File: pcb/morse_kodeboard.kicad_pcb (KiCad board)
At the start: 2 copper layers, 40 x 24 mm, 7 parts, among them J1 Conn_01x03, SW1 SW_DPST

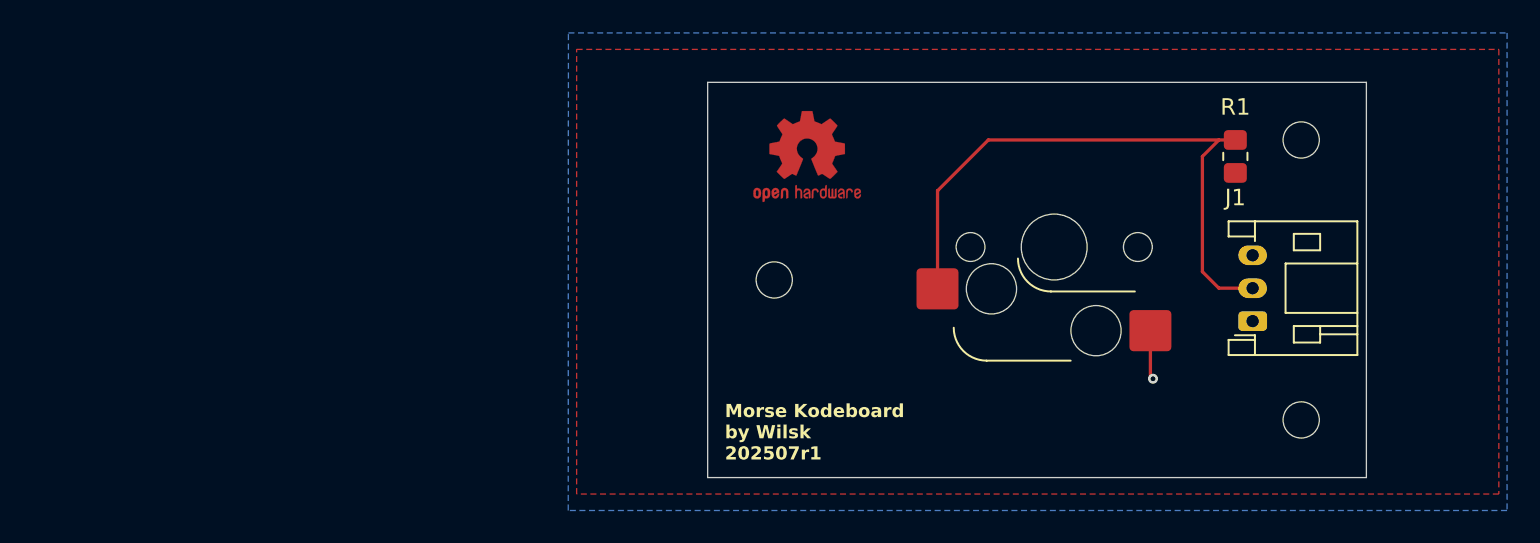
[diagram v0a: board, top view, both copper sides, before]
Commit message: Update PCB files with three buttons.
Sent off to fab as r1!

Signed-off-by: William Hart <391950+will-hart@users.noreply.github.com>
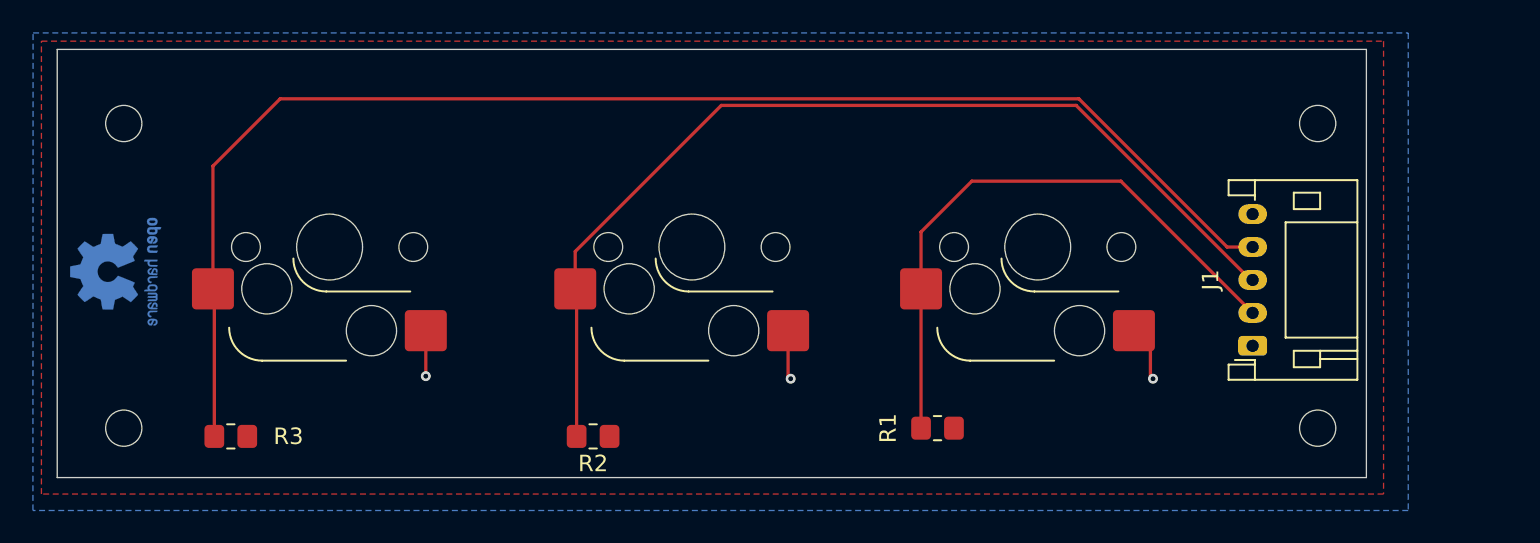
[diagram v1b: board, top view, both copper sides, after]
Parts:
- added H4: MountingHole, MountingHole:MountingHole_2.2mm_M2, F.Cu at (189.0, 43.5)
- added R2: R_US, Resistor_SMD:R_0805_2012Metric_Pad1.20x1.40mm_HandSolder, F.Cu at (145.0, 44.0)
- added R3: R_US, Resistor_SMD:R_0805_2012Metric_Pad1.20x1.40mm_HandSolder, F.Cu at (123.0, 44.0)
- added SW2: SW_DPST, PCM_Switch_Keyboard_Hotswap_Kailh:SW_Hotswap_Kailh_MX_1.00u, B.Cu at (151.0, 32.5)
- added SW3: SW_DPST, PCM_Switch_Keyboard_Hotswap_Kailh:SW_Hotswap_Kailh_MX_1.00u, B.Cu at (129.0, 32.5)
- J1: footprint Connector_JST:JST_PH_S3B-PH-K_1x03_P2.00mm_Horizontal -> Connector_JST:JST_PH_S5B-PH-K_1x05_P2.00mm_Horizontal
- SYM1: moved to B.Cu
- moved H2 71.5 mm to (116.5, 25.0)
- moved H3 71.5 mm to (116.5, 43.5)
- moved SYM1 42.6 mm to (116.0, 34.0), turned to -90 degrees
- moved H1 34.3 mm to (189.0, 25.0)
- moved R1 24.5 mm to (165.9, 43.5), turned to 180 degrees
- moved J1 1.50 mm to (185.1, 38.5)
- moved SW1 1.00 mm to (172.0, 32.5)
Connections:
- J1 pad 3: GND -> /SW2
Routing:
- net /SW3: track 0.00 -> 85.0 mm
- net /SW2: track 0.00 -> 60.5 mm
- net GND: track 2.99 -> 8.73 mm, vias 1 -> 3
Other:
- board size 40 x 24 mm -> 79.5 x 26 mm
- board text added: "G"
- board text added: "MORSE"
- board text added: "SHIFT"
- board text added: "SPACE"
- board text added: "V"
